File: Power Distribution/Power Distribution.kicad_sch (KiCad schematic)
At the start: 4 parts, among them SW1 SW_DPST_x2, U1 SC1176, U2 XL6009

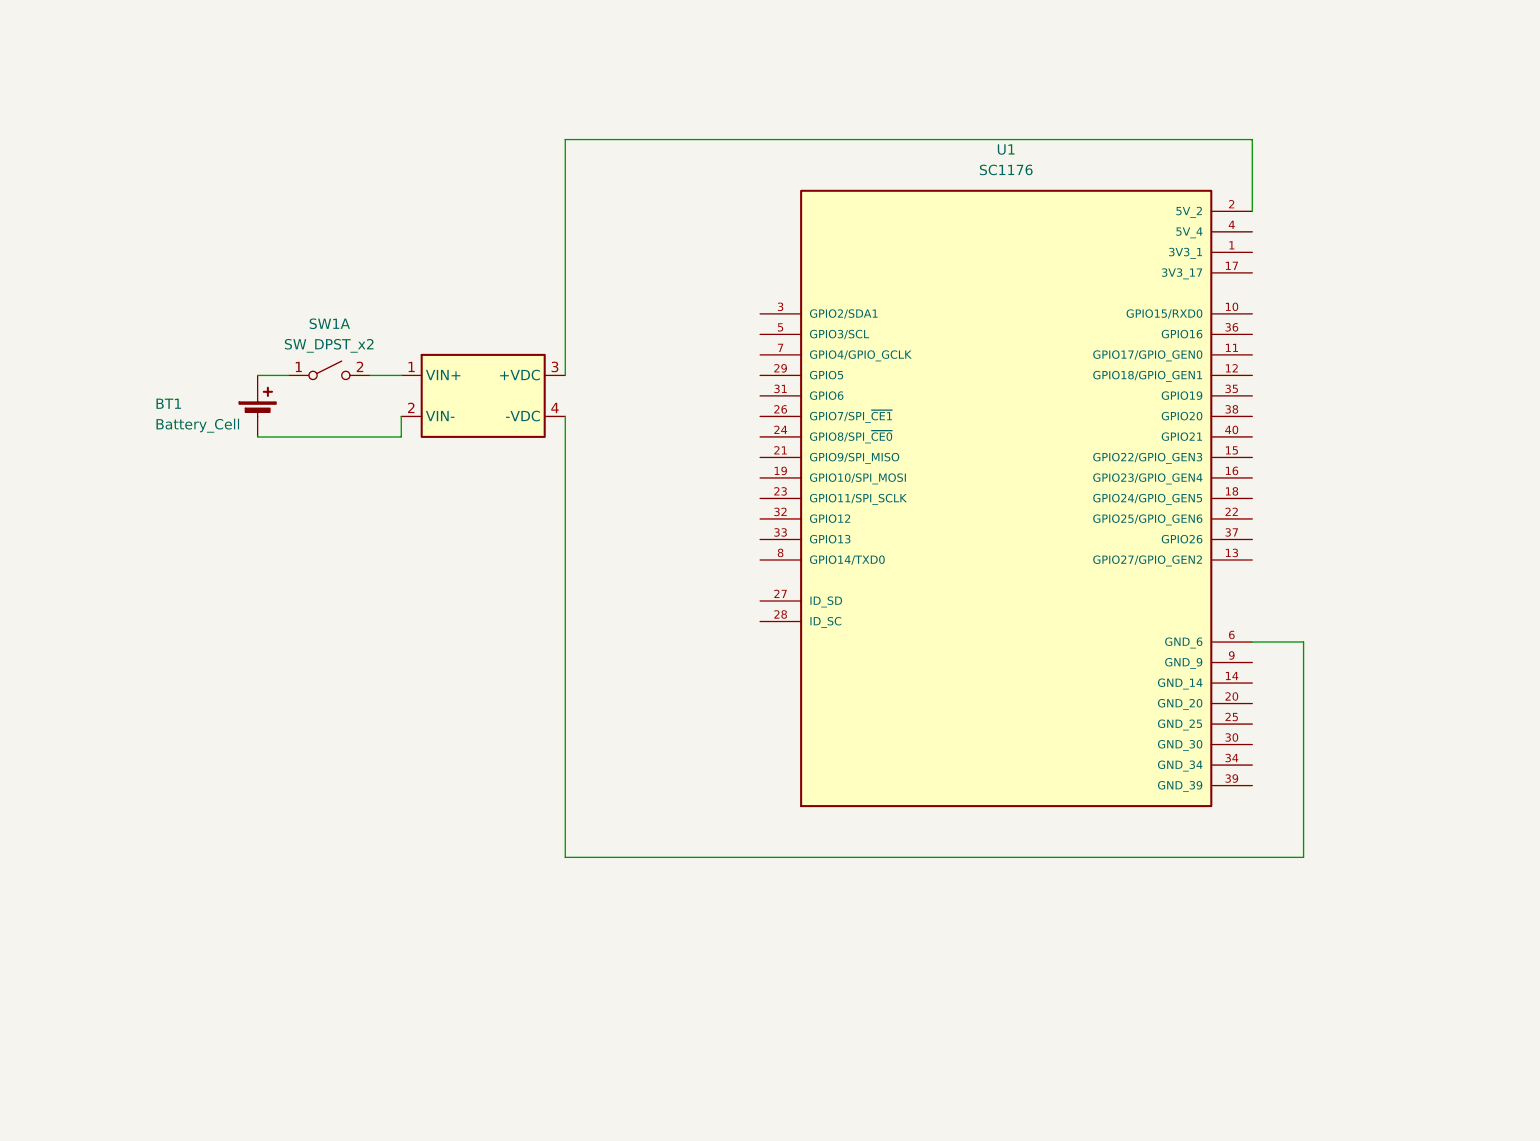
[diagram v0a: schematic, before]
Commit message: PCB
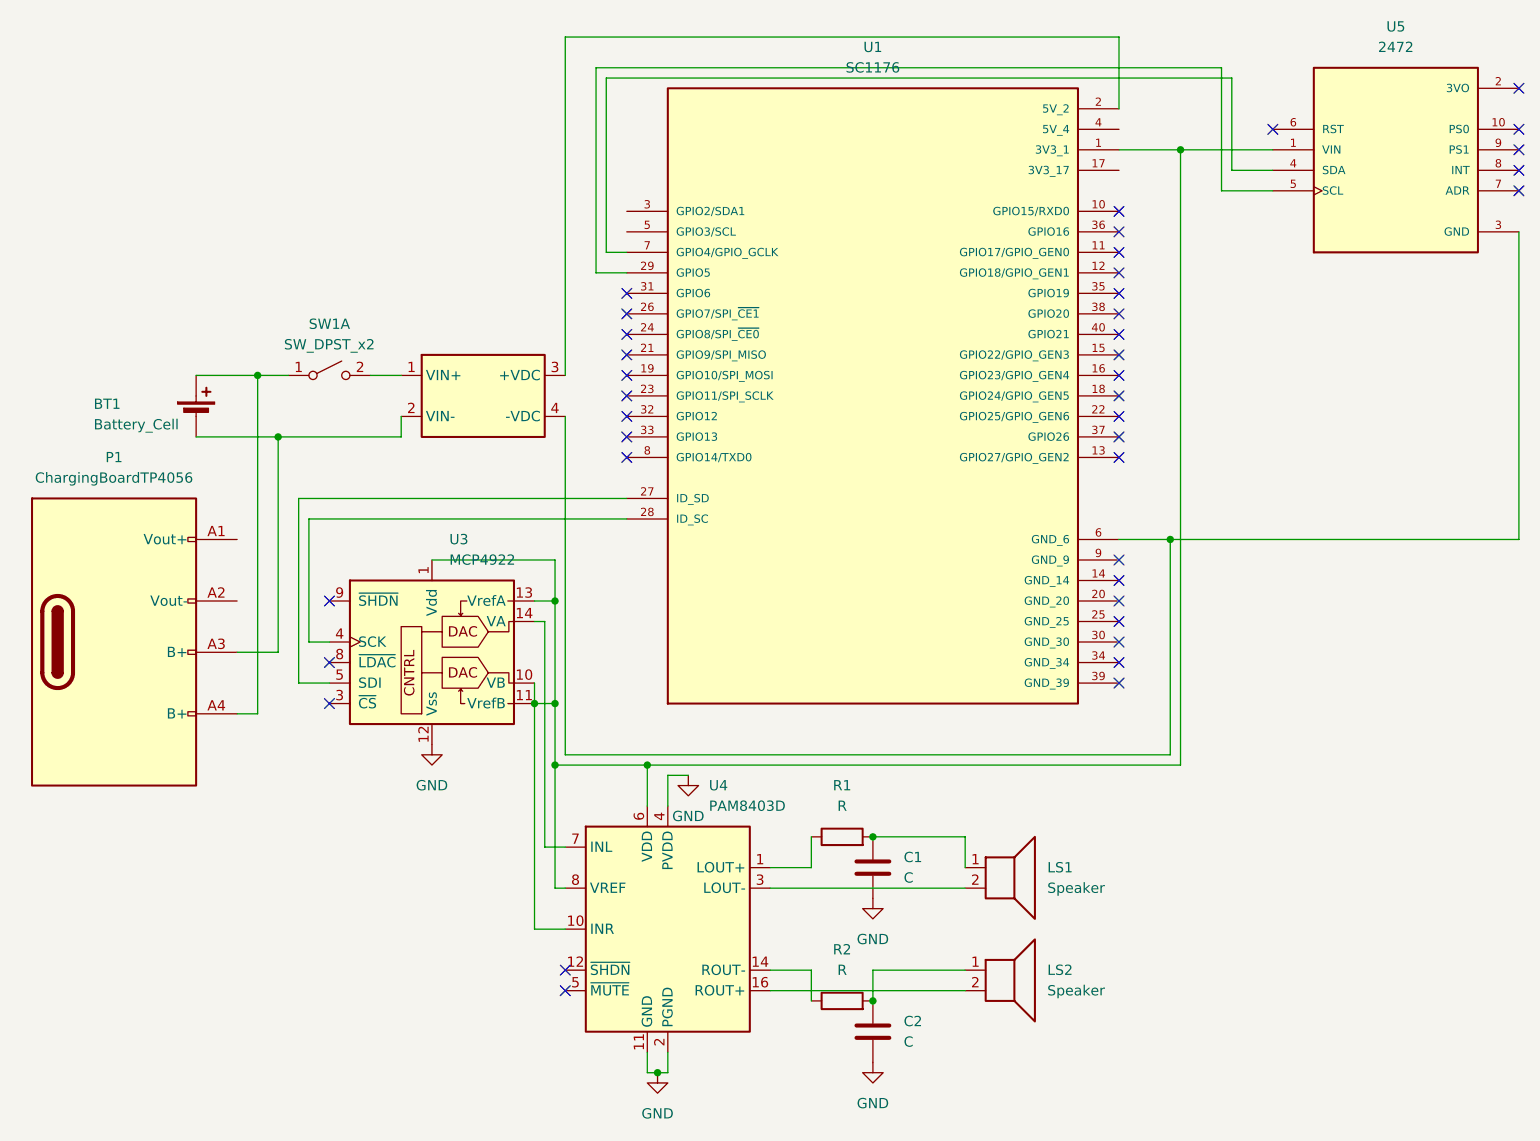
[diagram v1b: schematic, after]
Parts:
- added C1, C2: C, symbol Device:C
- added LS1, LS2: Speaker, symbol Device:Speaker
- added P1: ChargingBoardTP4056, symbol ChargingBoardTP4056:ChargingBoardTP4056
- added R1, R2: R, symbol Device:R
- added U3: MCP4922, symbol Analog_DAC:MCP4922
- added U4: PAM8403D, Package_SO:SOP-16_3.9x9.9mm_P1.27mm, symbol Amplifier_Audio:PAM8403D
- added U5: 2472, 2472:MODULE_2472, symbol 2472:2472
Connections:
- net at BT1.1 (+), SW1.1 (A): now also P1.A4 (B+)
- net at U1.1 (3V3_1): now also U3.1 (Vdd), U3.10 (VB), U3.11 (VrefB), U3.13 (VrefA), U4.10 (INR), U4.6 (VDD), U4.8 (VREF), U5.1 (VIN)
- net at U1.27 (ID_SD): now also U3.5 (SDI)
- net at U1.28 (ID_SC): now also U3.4 (SCK)
- net at U1.29 (GPIO5): now also U5.5 (SCL)
- net at U1.6 (GND_6), U2.4 (-VDC): now also U5.3 (GND)
- net at U1.7 (GPIO4/GPIO_GCLK): now also U5.4 (SDA)
- net at BT1.2 (-), U2.2 (+VDC), U2.8 (VIN-): now also P1.A3 (B+)
- new net: R1.1, U4.1 (LOUT+)
- new net: R2.1, U4.14 (ROUT-)
- new net: LS2.2, U4.16 (ROUT+)
- new net: LS1.2, U4.3 (LOUT-)
- new net: U3.14 (VA), U4.7 (INL)
- new net: C2.1, LS2.1, R2.2
- new net: C1.1, LS1.1, R1.2
- new net: P1.A1 (Vout+), P1.A9 (VBUS), P1.B4 (VBUS), P1.B9 (VBUS)
- new net GND: C1.2, C2.2, U3.12 (Vss), U4.11 (GND), U4.13 (PVDD), U4.15 (PGND), U4.2 (PGND), U4.4 (PVDD)
- no-connect marks 0 -> 40
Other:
- moved on the sheet: BT1, U1
